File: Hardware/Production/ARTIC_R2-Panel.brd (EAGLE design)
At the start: 113 x 122.2 mm, 1045 parts, among them J1 U.FL, J10 U.FL, J11 THING_PLUS, J12 U.FL, J13 THING_PLUS, J14 U.FL, J15 THING_PLUS, J16 U.FL, J2 THING_PLUS, J3 THING_PLUS, J4 U.FL, J5 THING_PLUS, J6 U.FL, J7 THING_PLUS, J8 U.FL, J9 THING_PLUS, Q1 20V/4.2A/52mΩ/1.4W, Q2 20V/4.2A/52mΩ/1.4W, Q3 20V/4.2A/52mΩ/1.4W, Q4 20V/4.2A/52mΩ/1.4W, Q5 20V/4.2A/52mΩ/1.4W, Q6 20V/4.2A/52mΩ/1.4W, Q7 20V/4.2A/52mΩ/1.4W, Q8 20V/4.2A/52mΩ/1.4W, U1 32M SPI Flash, U10 1.8V/100mA, U11 32M SPI Flash, U12 DUAL-OPTOISOLATOR_SOIC8, U13 ARTIC_R2, U14 RFPA0133, U15 AS179-92LF, U16 1.8V/100mA, U17 32M SPI Flash, U18 DUAL-OPTOISOLATOR_SOIC8, U19 ARTIC_R2, U2 1.8V/100mA, U20 RFPA0133, U21 AS179-92LF, U22 1.8V/100mA, U23 32M SPI Flash, U24 DUAL-OPTOISOLATOR_SOIC8, U25 ARTIC_R2, U26 RFPA0133, U27 AS179-92LF, U28 1.8V/100mA, U29 32M SPI Flash, U3 ARTIC_R2, U30 DUAL-OPTOISOLATOR_SOIC8, U31 ARTIC_R2, U32 RFPA0133, U33 AS179-92LF, U34 1.8V/100mA, U35 32M SPI Flash, U36 DUAL-OPTOISOLATOR_SOIC8, U37 ARTIC_R2, U38 RFPA0133, U39 AS179-92LF, U4 RFPA0133, U40 1.8V/100mA, U41 32M SPI Flash, U42 DUAL-OPTOISOLATOR_SOIC8, U43 ARTIC_R2, U44 RFPA0133, U45 AS179-92LF, U46 1.8V/100mA, U47 32M SPI Flash, U48 DUAL-OPTOISOLATOR_SOIC8, U5 AS179-92LF, U6 DUAL-OPTOISOLATOR_SOIC8, U7 ARTIC_R2, U8 RFPA0133, U9 AS179-92LF, X1 CRYSTAL-TCXO-26MHZ, X2 CRYSTAL-TCXO-26MHZ, X3 CRYSTAL-TCXO-26MHZ, X4 CRYSTAL-TCXO-26MHZ, X5 CRYSTAL-TCXO-26MHZ, X6 CRYSTAL-TCXO-26MHZ, X7 CRYSTAL-TCXO-26MHZ, X8 CRYSTAL-TCXO-26MHZ

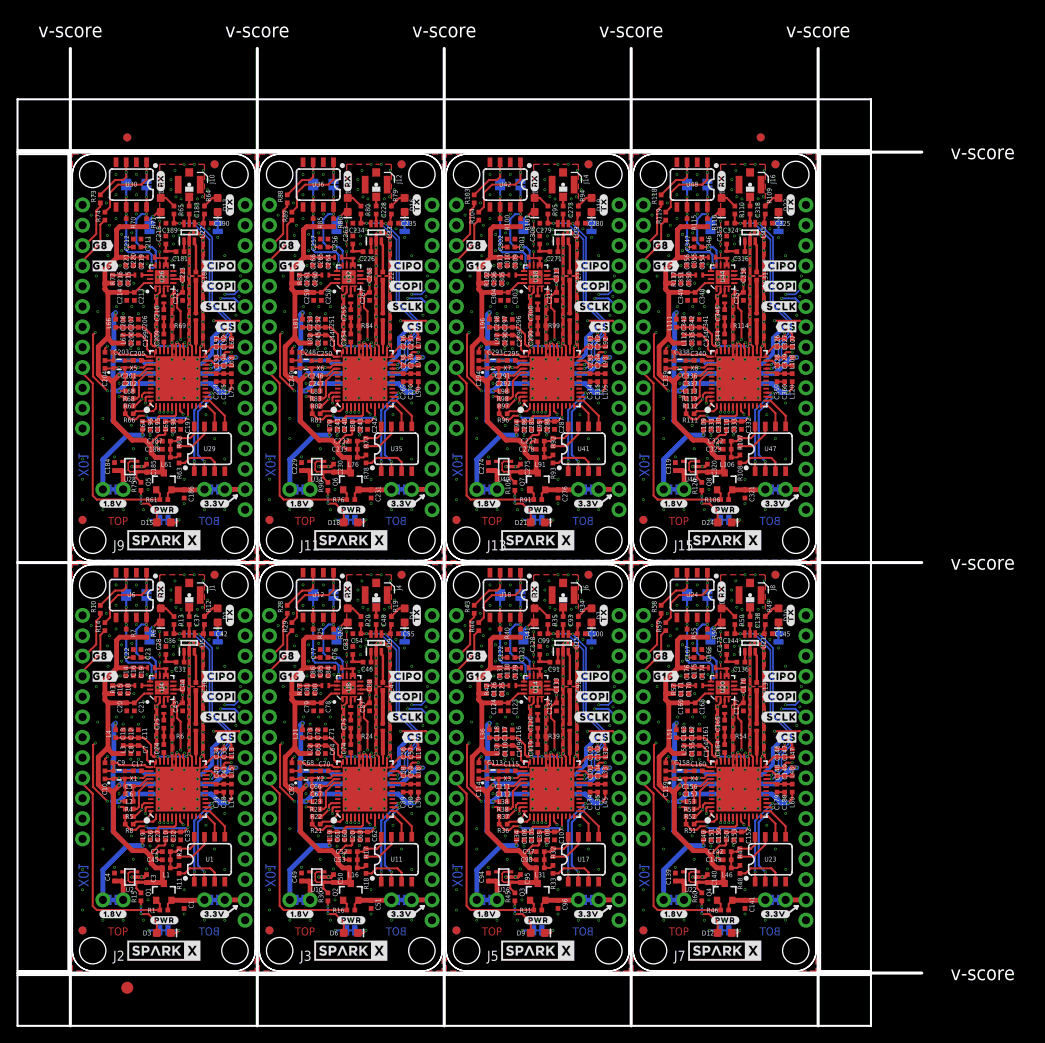
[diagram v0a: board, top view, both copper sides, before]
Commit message: Updates for X02
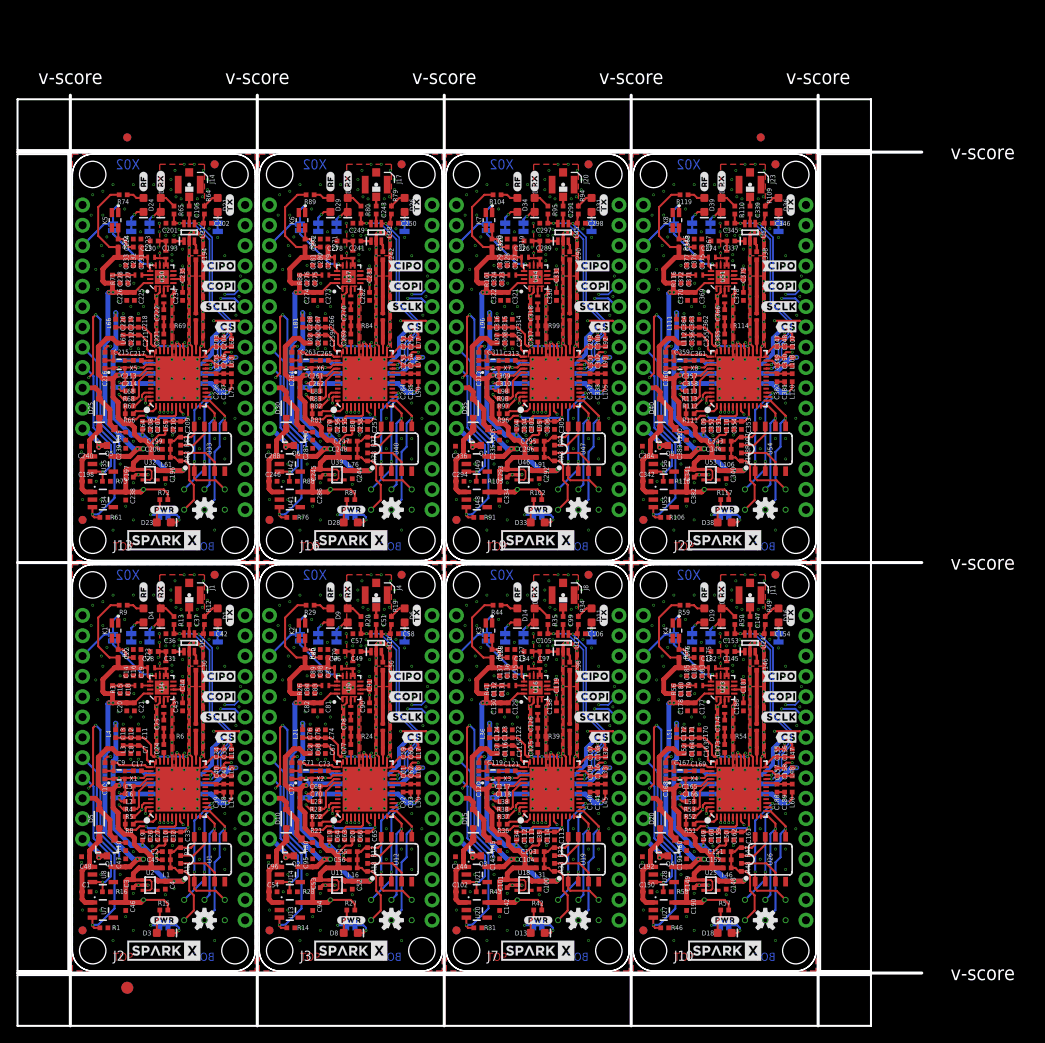
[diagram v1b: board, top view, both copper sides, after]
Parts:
- removed JP41, JP42, JP48, JP49, JP55, JP56: JUMPER-SMT_2_NO_SILK, SparkFun-Jumpers:SMT-JUMPER_2_NO_SILK
- removed JP43, JP44, JP50, JP51: JUMPER-COMBO_2_NC_TRACE, SparkFun-Jumpers:COMBO-JUMPER_2_NC_TRACE
- removed JP45, JP46, JP47, JP52, JP53, JP54: JUMPER-SMT_2_NC_TRACE_SILK, SparkFun-Jumpers:SMT-JUMPER_2_NC_TRACE_SILK
- removed U$225: (no value), output:#RESETB0
- removed U$226: (no value), output:#PWR_EN0
- removed U$227: (no value), output:GND#0
- removed U$228: (no value), output:#INT20
- removed U$229: (no value), output:#INT10
- removed U$230: (no value), output:#PWR_LED#0
- removed U$231: (no value), output:#PWR#0
- removed U$232: (no value), output:ARTIC_R2_BREAKOUT0
- added C361: 1.0nF, SparkFun-Capacitors:0402-TIGHT
- added C362, C365, C366, C367, C368, C369, C375, C378: 100pF, SparkFun-Capacitors:0402-TIGHT
- added C363: 1.0uF, SparkFun-Capacitors:0402-TIGHT
- added C364, C377: 10uF, SparkFun-Capacitors:0402-TIGHT
- added C370, C372, C376, C379, C382, C383: 2.2uF, SparkFun-Capacitors:0402-TIGHT
- added C371, C380: 22pF, SparkFun-Capacitors:0402-TIGHT
- added C373: 2.4 pF, SparkFun-Capacitors:0402_MURATA
- added C374: 9.1pF, New_Parts_Capacitors:0402-TIGHT
- added C381, C384: 0.1uF, SparkFun-Capacitors:0402-TIGHT
- added D25, D30, D35, D40: 1A/23V/620mV, SparkFun-DiscreteSemi:SOD-323
- added D26, D27, D31, D32, D36, D37: Yellow, SparkFun-LED:LED-0603
- added D28, D29, D33, D34, D38, D39: RED, SparkFun-LED:LED-0603
- added E$6: (no value), SparkFun-Retired:FIDUCIAL-1.5X3
- added J17, J20, J23: U.FL, SparkFun-Connectors:U.FL
- added J18, J21, J24: Flash Programming, SparkFun-Connectors:2X3_TEST_POINTS
- added J19, J22: THING_PLUS, New_Parts_Boards:THING_PLUS
- added K1, K2, K3, K4, K5, K6, K7, K8: TLP3475R, New_Parts_DiscreteSemi:TLP3475RTPF
- added LOGO1, LOGO10, LOGO11, LOGO12, LOGO13, LOGO14, LOGO15, LOGO16, LOGO2, LOGO3, LOGO4, LOGO5, LOGO6, LOGO7, LOGO8, LOGO9: OSHW-LOGOS, SparkFun-Aesthetics:OSHW-LOGO-S
- added TP1, TP10, TP11, TP12, TP13, TP14, TP15, TP16, TP17, TP18, TP19, TP2, TP20, TP21, TP22, TP23, TP24, TP3, TP4, TP5, TP6, TP7, TP8, TP9: TEST-POINTTP_15TH_THRU, SparkFun-Connectors:TP_15TH
- added U49, U55, U56: 3.3V, SparkFun-IC-Power:SOT23-5
- added U50: ARTIC_R2, New_Parts_IC-Comms:QFN-48
- added U51: RFPA0133, New_Parts_IC-Comms:QFN50P300X300X86-17N
- added U52: AS179-92LF, New_Parts_IC-Comms:SOT65P220X100-6N
- added U53: 1.8V/100mA, SparkFun-IC-Power:SC70
- added U54: 2Mbit SPI Flash, New_Parts_IC-Memory:SO08
- C1, C276: value 10uF -> 2.2uF
- C100, C119, C123, C167, C219, C267, C341, C71, C75: value 100pF -> 1.0uF
- C101, C148, C197, C215, C244, C359, C52: value 22pF -> 1.0uF
- C102, C143, C180, C198, C239, C286, C331, C335: value 0.1uF -> 2.2uF
- C105, C125, C146, C154, C170, C193, C195, C201, C224, C242, C269, C289, C291, C314, C330, C58, C80, C97: value 22pF -> 100pF
- C106, C135, C147, C153, C194, C202, C225, C241, C243, C270, C282, C290, C327, C337, C57, C90, C98: value 0.1uF -> 100pF
- C113, C117, C140, C203, C207, C275: value 1.0uF -> 22pF
- C114, C204: value 47nF -> 0.1uF
- C115, C205, C295: value 1.0nF -> 22pF
- C116, C144, C164, C166, C189, C206, C210, C212, C254, C256, C258, C296, C300, C302, C344, C348, C354, C48, C93: value 100pF -> 0.1uF
- C118, C141, C208, C356, C96: value 10uF -> 0.1uF
- C120, C168, C264, C312: value 100pF -> 47nF
- C121: value 100pF -> 1.0nF
- C124, C220, C268: value 2.2uF -> 10uF
- C126, C175, C223, C79, C81: value 2.2uF -> 100pF
- C127: value 2.4 pF -> 100pF; device SparkFun-Capacitors:0402_MURATA -> SparkFun-Capacitors:0402-TIGHT
- C128, C173, C218: value 9.1pF -> 100pF; device New_Parts_Capacitors:0402-TIGHT -> SparkFun-Capacitors:0402-TIGHT
- C131, C163, C253, C343: value 10uF -> 22pF
- C132, C136, C190, C226, C228, C235, C280, C324, C46, C47, C54, C84, C91: value 100pF -> 2.2uF
- C133, C85: value 2.2uF -> 2.4 pF; device SparkFun-Capacitors:0402-TIGHT -> SparkFun-Capacitors:0402_MURATA
- C134, C326: value 22pF -> 9.1pF; device SparkFun-Capacitors:0402-TIGHT -> New_Parts_Capacitors:0402-TIGHT
- C137, C316, C76: value 100pF -> 10uF
- C139, C184, C274, C342, C94, C95: value 1.0uF -> 2.2uF
- C142, C150, C187, C191, C232, C238, C246, C283, C287, C322, C328, C334: value 22pF -> 2.2uF
- C149, C196, C245, C292, C315, C53: value 0.1uF -> 1.0uF
- C151, C155, C157, C188, C247, C284, C323, C59, C61, C63, C65, C67: value 0.1uF -> 22pF
- C152, C156, C240, C260, C285, C336, C350, C56, C60, C62, C64, C66: value 22pF -> 0.1uF
- C158, C162, C248, C252, C68: value 1.0uF -> 0.1uF
- C159, C69: value 47nF -> 22pF
- C160, C70: value 1.0nF -> 0.1uF
- C161, C165, C209, C211, C213, C227, C251, C255, C257, C299, C301, C303, C309, C347, C357, C55, C92: value 100pF -> 22pF
- C169, C265, C313: value 2.2uF -> 1.0nF
- C171: value 2.2uF -> 1.0uF
- C172: value 2.4 pF -> 10uF; device SparkFun-Capacitors:0402_MURATA -> SparkFun-Capacitors:0402-TIGHT
- C176, C186, C221, C231, C266, C298, C321, C51: value 10uF -> 100pF
- C181, C325: value 100pF -> 2.4 pF; device SparkFun-Capacitors:0402-TIGHT -> SparkFun-Capacitors:0402_MURATA
- C182: value 100pF -> 9.1pF; device SparkFun-Capacitors:0402-TIGHT -> New_Parts_Capacitors:0402-TIGHT
- C185: value 1.0uF -> 10uF
- C214, C304, C306, C310, C358: value 2.2uF -> 0.1uF
- C216: value 2.2uF -> 47nF
- C217: value 2.4 pF -> 1.0nF; device SparkFun-Capacitors:0402_MURATA -> SparkFun-Capacitors:0402-TIGHT
- C229: value 1.0uF -> 2.4 pF; device SparkFun-Capacitors:0402-TIGHT -> SparkFun-Capacitors:0402_MURATA
- C230: value 1.0uF -> 9.1pF; device SparkFun-Capacitors:0402-TIGHT -> New_Parts_Capacitors:0402-TIGHT
- C233, C329: value 0.1uF -> 10uF
- C249, C339: value 47nF -> 100pF
- C250: value 1.0nF -> 100pF
- C259, C261, C349, C351, C355: value 2.2uF -> 22pF
- C262, C352: value 2.4 pF -> 0.1uF; device SparkFun-Capacitors:0402_MURATA -> SparkFun-Capacitors:0402-TIGHT
- C263: value 9.1pF -> 1.0uF; device New_Parts_Capacitors:0402-TIGHT -> SparkFun-Capacitors:0402-TIGHT
- C277: value 22pF -> 2.4 pF; device SparkFun-Capacitors:0402-TIGHT -> SparkFun-Capacitors:0402_MURATA
- C278: value 0.1uF -> 9.1pF; device SparkFun-Capacitors:0402-TIGHT -> New_Parts_Capacitors:0402-TIGHT
- C281, C89: value 22pF -> 10uF
- C294: value 47nF -> 2.2uF
- C297, C319, C320, C338, C49, C50: value 1.0uF -> 100pF
- C307: value 2.4 pF -> 22pF; device SparkFun-Capacitors:0402_MURATA -> SparkFun-Capacitors:0402-TIGHT
- C308: value 9.1pF -> 0.1uF; device New_Parts_Capacitors:0402-TIGHT -> SparkFun-Capacitors:0402-TIGHT
- C311: value 10uF -> 1.0uF
- C340: value 1.0nF -> 1.0uF
- C353, C83: value 9.1pF -> 22pF; device New_Parts_Capacitors:0402-TIGHT -> SparkFun-Capacitors:0402-TIGHT
- C360: value 0.1uF -> 47nF
- C72: value 1.0uF -> 47nF
- C73: value 10uF -> 1.0nF
- C82: value 2.4 pF -> 2.2uF; device SparkFun-Capacitors:0402_MURATA -> SparkFun-Capacitors:0402-TIGHT
- C86: value 10uF -> 9.1pF; device SparkFun-Capacitors:0402-TIGHT -> New_Parts_Capacitors:0402-TIGHT
- D10, D20, D5: value Yellow -> 1A/23V/620mV; device SparkFun-LED:LED-0603 -> SparkFun-DiscreteSemi:SOD-323
- D12, D21, D6: value RED -> Yellow
- D13, D14, D19, D23, D4, D8: value Yellow -> RED
- D15: value RED -> 1A/23V/620mV; device SparkFun-LED:LED-0603 -> SparkFun-DiscreteSemi:SOD-323
- J10, J16: value U.FL -> THING_PLUS; device SparkFun-Connectors:U.FL -> New_Parts_Boards:THING_PLUS
- J11: value THING_PLUS -> U.FL; device New_Parts_Boards:THING_PLUS -> SparkFun-Connectors:U.FL
- J12, J6: value U.FL -> Flash Programming; device SparkFun-Connectors:U.FL -> SparkFun-Connectors:2X3_TEST_POINTS
- J15, J5, J9: value THING_PLUS -> Flash Programming; device New_Parts_Boards:THING_PLUS -> SparkFun-Connectors:2X3_TEST_POINTS
- JP1, JP15, JP16, JP2, JP22, JP23, JP30, JP36, JP37, JP8: value JUMPER-COMBO_2_NC_TRACE -> JUMPER-SMT_2_NC_TRACE_SILK; device SparkFun-Jumpers:COMBO-JUMPER_2_NC_TRACE -> SparkFun-Jumpers:SMT-JUMPER_2_NC_TRACE_SILK
- JP13, JP20, JP21, JP27, JP28, JP35, JP6: value JUMPER-SMT_2_NO_SILK -> JUMPER-SMT_2_NC_TRACE_SILK; device SparkFun-Jumpers:SMT-JUMPER_2_NO_SILK -> SparkFun-Jumpers:SMT-JUMPER_2_NC_TRACE_SILK
- JP19, JP24, JP39: value JUMPER-SMT_2_NC_TRACE_SILK -> JUMPER-SMT_2_NO_SILK; device SparkFun-Jumpers:SMT-JUMPER_2_NC_TRACE_SILK -> SparkFun-Jumpers:SMT-JUMPER_2_NO_SILK
- JP29, JP9: value JUMPER-COMBO_2_NC_TRACE -> JUMPER-SMT_2_NO_SILK; device SparkFun-Jumpers:COMBO-JUMPER_2_NC_TRACE -> SparkFun-Jumpers:SMT-JUMPER_2_NO_SILK
- Q1, Q2, Q3, Q4, Q5, Q6, Q7, Q8: value 20V/4.2A/52mΩ/1.4W -> 3.1A/30V/105mΩ
- R10, R103, R105, R118, R120, R14, R28, R30, R43, R45, R58, R60, R73, R75, R88, R90: value 1k -> 100k
- R100, R115, R25, R40, R55, R7, R70, R85: value 100k -> 10k
- R101, R116, R26, R41, R56, R71, R86: value 100k -> 3.9OHM; device SparkFun-Resistors:0402-TIGHT -> New_Parts_Resistors:0402-TIGHT
- R102, R117, R27, R42, R57, R72, R87: value 3.9OHM -> 1k; device New_Parts_Resistors:0402-TIGHT -> SparkFun-Resistors:0402-TIGHT
- R9: value 100k -> 1k
- U$100: device output:#SCLK0 -> output:GND#0
- U$101: device output:SCLK#0 -> output:#INT20
- U$102: device output:#CS0 -> output:#INT10
- U$103: device output:CS#0 -> output:#PWR_LED#0
- U$104: device output:G8#0 -> output:#PWR#0
- U$105: device output:#G80 -> output:ARTIC_R2_BREAKOUT0
- U$106: device output:G16#0 -> output:#RF_LED#0
- U$107: device output:#G160 -> output:#GAIN8#0
- U$108: device output:#BOOT0 -> output:#RF#0
- U$109: device output:#RESETB0 -> output:#RF_EN#0
- U$110: device output:#PWR_EN0 -> output:#VBATT#0
- U$111: device output:GND#0 -> output:##8DB#0
- U$112: device output:#INT20 -> output:#VUSB#0
- U$113: device output:#INT10 -> output:#RX_LED#0
- U$114: device output:#PWR_LED#0 -> output:#TX_LED#0
- U$115: device output:#PWR#0 -> output:#TX#0
- U$116: device output:ARTIC_R2_BREAKOUT0 -> output:#RX#0
- U$117: device output:#RX_LED#0 -> output:CIPO#0
- U$118: device output:#TX_LED#0 -> output:#CIPO0
- U$119, U$91: device output:#3#3V#0 -> output:#COPI0
- U$120, U$148: device output:#3#3V#0 -> output:COPI#0
- U$121, U$93: device output:#1#8V#0 -> output:#SCLK0
- U$122, U$150: device output:#1#8V#0 -> output:SCLK#0
- U$123: device output:#TX#0 -> output:#CS0
- U$124: device output:#RX#0 -> output:CS#0
- U$125: device output:CIPO#0 -> output:#BOOT0
- U$126: device output:#CIPO0 -> output:#RESETB0
- U$127: device output:#COPI0 -> output:#PWR_EN0
- U$128: device output:COPI#0 -> output:GND#0
- U$129: device output:#SCLK0 -> output:#INT20
- U$130: device output:SCLK#0 -> output:#INT10
- U$131: device output:#CS0 -> output:#PWR_LED#0
- U$132: device output:CS#0 -> output:#PWR#0
- U$133: device output:G8#0 -> output:ARTIC_R2_BREAKOUT0
- U$134: device output:#G80 -> output:#RF_LED#0
- U$135: device output:G16#0 -> output:#GAIN8#0
- U$136: device output:#G160 -> output:#RF#0
- U$137: device output:#BOOT0 -> output:#RF_EN#0
- U$138: device output:#RESETB0 -> output:#VBATT#0
- U$139: device output:#PWR_EN0 -> output:##8DB#0
- U$140: device output:GND#0 -> output:#VUSB#0
- U$141: device output:#INT20 -> output:#RX_LED#0
- U$142: device output:#INT10 -> output:#TX_LED#0
- U$143: device output:#PWR_LED#0 -> output:#TX#0
- U$144: device output:#PWR#0 -> output:#RX#0
- U$145: device output:ARTIC_R2_BREAKOUT0 -> output:CIPO#0
- U$146: device output:#RX_LED#0 -> output:#CIPO0
- U$147: device output:#TX_LED#0 -> output:#COPI0
- U$149, U$177: device output:#3#3V#0 -> output:#SCLK0
- U$151, U$179: device output:#1#8V#0 -> output:#CS0
- U$152: device output:#TX#0 -> output:CS#0
- U$153: device output:#RX#0 -> output:#BOOT0
- U$154: device output:CIPO#0 -> output:#RESETB0
- U$155: device output:#CIPO0 -> output:#PWR_EN0
- U$156: device output:#COPI0 -> output:GND#0
- U$157: device output:COPI#0 -> output:#INT20
- U$158: device output:#SCLK0 -> output:#INT10
- U$159: device output:SCLK#0 -> output:#PWR_LED#0
- U$160: device output:#CS0 -> output:#PWR#0
- U$161: device output:CS#0 -> output:ARTIC_R2_BREAKOUT0
- U$162: device output:G8#0 -> output:#RF_LED#0
- U$163: device output:#G80 -> output:#GAIN8#0
- U$164: device output:G16#0 -> output:#RF#0
- U$165: device output:#G160 -> output:#RF_EN#0
- U$166: device output:#BOOT0 -> output:#VBATT#0
- U$167: device output:#RESETB0 -> output:##8DB#0
- U$168: device output:#PWR_EN0 -> output:#VUSB#0
- U$169: device output:GND#0 -> output:#RX_LED#0
- U$170: device output:#INT20 -> output:#TX_LED#0
- U$171: device output:#INT10 -> output:#TX#0
- U$172: device output:#PWR_LED#0 -> output:#RX#0
- U$173: device output:#PWR#0 -> output:CIPO#0
- U$174: device output:ARTIC_R2_BREAKOUT0 -> output:#CIPO0
- U$175: device output:#RX_LED#0 -> output:#COPI0
- U$176: device output:#TX_LED#0 -> output:COPI#0
- U$178, U$206: device output:#3#3V#0 -> output:SCLK#0
- U$180, U$208: device output:#1#8V#0 -> output:CS#0
- U$181: device output:#TX#0 -> output:#BOOT0
- U$182: device output:#RX#0 -> output:#RESETB0
- U$183: device output:CIPO#0 -> output:#PWR_EN0
- U$184: device output:#CIPO0 -> output:GND#0
- U$185: device output:#COPI0 -> output:#INT20
- U$186: device output:COPI#0 -> output:#INT10
- U$187: device output:#SCLK0 -> output:#PWR_LED#0
- U$188: device output:SCLK#0 -> output:#PWR#0
- U$189: device output:#CS0 -> output:ARTIC_R2_BREAKOUT0
- U$190: device output:CS#0 -> output:#RF_LED#0
- U$191: device output:G8#0 -> output:#GAIN8#0
- U$192: device output:#G80 -> output:#RF#0
- U$193: device output:G16#0 -> output:#RF_EN#0
- U$194: device output:#G160 -> output:#VBATT#0
- U$195: device output:#BOOT0 -> output:##8DB#0
- U$196: device output:#RESETB0 -> output:#VUSB#0
- U$197: device output:#PWR_EN0 -> output:#RX_LED#0
- U$198: device output:GND#0 -> output:#TX_LED#0
- U$199: device output:#INT20 -> output:#TX#0
- U$20: device output:G8#0 -> output:#VBATT#0
- U$200: device output:#INT10 -> output:#RX#0
- U$201: device output:#PWR_LED#0 -> output:CIPO#0
- U$202: device output:#PWR#0 -> output:#CIPO0
- U$203: device output:ARTIC_R2_BREAKOUT0 -> output:#COPI0
- U$204: device output:#RX_LED#0 -> output:COPI#0
- U$205: device output:#TX_LED#0 -> output:#SCLK0
- U$207: device output:#3#3V#0 -> output:#CS0
- U$209: device output:#1#8V#0 -> output:#BOOT0
- U$21: device output:#G80 -> output:#VUSB#0
- U$210: device output:#TX#0 -> output:#RESETB0
- U$211: device output:#RX#0 -> output:#PWR_EN0
- U$212: device output:CIPO#0 -> output:GND#0
- U$213: device output:#CIPO0 -> output:#INT20
- U$214: device output:#COPI0 -> output:#INT10
- U$215: device output:COPI#0 -> output:#PWR_LED#0
- U$216: device output:#SCLK0 -> output:#PWR#0
- U$217: device output:SCLK#0 -> output:ARTIC_R2_BREAKOUT0
- U$218: device output:#CS0 -> output:#RF_LED#0
- U$219: device output:CS#0 -> output:#GAIN8#0
- U$22: device output:G16#0 -> output:##8DB#0
- U$220: device output:G8#0 -> output:#RF#0
- U$221: device output:#G80 -> output:#RF_EN#0
- U$222: device output:G16#0 -> output:#VBATT#0
- U$223: device output:#G160 -> output:##8DB#0
- U$224: device output:#BOOT0 -> output:#VUSB#0
- U$23: device output:#G160 -> output:#RX_LED#0
- U$30: device output:#RX_LED#0 -> output:#TX_LED#0
- U$31: device output:#TX_LED#0 -> output:#TX#0
- U$32: device output:#3#3V#0 -> output:#RX#0
- U$33, U$61: device output:#3#3V#0 -> output:CIPO#0
- U$34: device output:#1#8V#0 -> output:#CIPO0
- U$35, U$63: device output:#1#8V#0 -> output:#COPI0
- U$36: device output:#TX#0 -> output:COPI#0
- U$37: device output:#RX#0 -> output:#SCLK0
- U$38: device output:CIPO#0 -> output:SCLK#0
- U$39: device output:#CIPO0 -> output:#CS0
- U$40: device output:#COPI0 -> output:CS#0
- U$41: device output:COPI#0 -> output:#BOOT0
- U$42: device output:#SCLK0 -> output:#RESETB0
- U$43: device output:SCLK#0 -> output:#PWR_EN0
- U$44: device output:#CS0 -> output:GND#0
- U$45: device output:CS#0 -> output:#INT20
- U$46: device output:G8#0 -> output:#INT10
- U$47: device output:#G80 -> output:#PWR_LED#0
- U$48: device output:G16#0 -> output:#PWR#0
- U$49: device output:#G160 -> output:ARTIC_R2_BREAKOUT0
- U$5: device output:#3#3V#0 -> output:#RF_LED#0
- U$50: device output:#BOOT0 -> output:#RF_LED#0
- U$51: device output:#RESETB0 -> output:#GAIN8#0
- U$52: device output:#PWR_EN0 -> output:#RF#0
- U$53: device output:GND#0 -> output:#RF_EN#0
- U$54: device output:#INT20 -> output:#VBATT#0
- U$55: device output:#INT10 -> output:##8DB#0
- U$56: device output:#PWR_LED#0 -> output:#VUSB#0
- U$57: device output:#PWR#0 -> output:#RX_LED#0
- U$58: device output:ARTIC_R2_BREAKOUT0 -> output:#TX_LED#0
- U$59: device output:#RX_LED#0 -> output:#TX#0
- U$6: device output:#3#3V#0 -> output:#GAIN8#0
- U$60: device output:#TX_LED#0 -> output:#RX#0
- U$62, U$90: device output:#3#3V#0 -> output:#CIPO0
- U$64, U$92: device output:#1#8V#0 -> output:COPI#0
- U$65: device output:#TX#0 -> output:#SCLK0
- U$66: device output:#RX#0 -> output:SCLK#0
- U$67: device output:CIPO#0 -> output:#CS0
- U$68: device output:#CIPO0 -> output:CS#0
- U$69: device output:#COPI0 -> output:#BOOT0
- U$7: device output:#1#8V#0 -> output:#RF#0
- U$70: device output:COPI#0 -> output:#RESETB0
- U$71: device output:#SCLK0 -> output:#PWR_EN0
- U$72: device output:SCLK#0 -> output:GND#0
- U$73: device output:#CS0 -> output:#INT20
- U$74: device output:CS#0 -> output:#INT10
- U$75: device output:G8#0 -> output:#PWR_LED#0
- U$76: device output:#G80 -> output:#PWR#0
- U$77: device output:G16#0 -> output:ARTIC_R2_BREAKOUT0
- U$78: device output:#G160 -> output:#RF_LED#0
- U$79: device output:#BOOT0 -> output:#GAIN8#0
- U$8: device output:#1#8V#0 -> output:#RF_EN#0
- U$80: device output:#RESETB0 -> output:#RF#0
- U$81: device output:#PWR_EN0 -> output:#RF_EN#0
- U$82: device output:GND#0 -> output:#VBATT#0
- U$83: device output:#INT20 -> output:##8DB#0
- U$84: device output:#INT10 -> output:#VUSB#0
- U$85: device output:#PWR_LED#0 -> output:#RX_LED#0
- U$86: device output:#PWR#0 -> output:#TX_LED#0
- U$87: device output:ARTIC_R2_BREAKOUT0 -> output:#TX#0
- U$88: device output:#RX_LED#0 -> output:#RX#0
- U$89: device output:#TX_LED#0 -> output:CIPO#0
- U$94: device output:#TX#0 -> output:SCLK#0
- U$95: device output:#RX#0 -> output:#CS0
- U$96: device output:CIPO#0 -> output:CS#0
- U$97: device output:#CIPO0 -> output:#BOOT0
- U$98: device output:#COPI0 -> output:#RESETB0
- U$99: device output:COPI#0 -> output:#PWR_EN0
- U1, U47: value 32M SPI Flash -> 2Mbit SPI Flash; device SparkFun-IC-Memory:SO08 -> New_Parts_IC-Memory:SO08
- U10: value 1.8V/100mA -> AS179-92LF; device SparkFun-IC-Power:SC70 -> New_Parts_IC-Comms:SOT65P220X100-6N
- U11: value 32M SPI Flash -> 1.8V/100mA; device SparkFun-IC-Memory:SO08 -> SparkFun-IC-Power:SC70
- U12: value DUAL-OPTOISOLATOR_SOIC8 -> 2Mbit SPI Flash; device SparkFun-DiscreteSemi:SO08 -> New_Parts_IC-Memory:SO08
- U13, U7: value ARTIC_R2 -> 3.3V; device New_Parts_IC-Comms:QFN-48 -> SparkFun-IC-Power:SOT23-5
- U14, U20, U8: value RFPA0133 -> 3.3V; device New_Parts_IC-Comms:QFN50P300X300X86-17N -> SparkFun-IC-Power:SOT23-5
- U15: value AS179-92LF -> ARTIC_R2; device New_Parts_IC-Comms:SOT65P220X100-6N -> New_Parts_IC-Comms:QFN-48
- U16: value 1.8V/100mA -> RFPA0133; device SparkFun-IC-Power:SC70 -> New_Parts_IC-Comms:QFN50P300X300X86-17N
- U17: value 32M SPI Flash -> AS179-92LF; device SparkFun-IC-Memory:SO08 -> New_Parts_IC-Comms:SOT65P220X100-6N
- U18: value DUAL-OPTOISOLATOR_SOIC8 -> 1.8V/100mA; device SparkFun-DiscreteSemi:SO08 -> SparkFun-IC-Power:SC70
- U19: value ARTIC_R2 -> 2Mbit SPI Flash; device New_Parts_IC-Comms:QFN-48 -> New_Parts_IC-Memory:SO08
- U21, U27: value AS179-92LF -> 3.3V; device New_Parts_IC-Comms:SOT65P220X100-6N -> SparkFun-IC-Power:SOT23-5
- U22: value 1.8V/100mA -> ARTIC_R2; device SparkFun-IC-Power:SC70 -> New_Parts_IC-Comms:QFN-48
- U23: value 32M SPI Flash -> RFPA0133; device SparkFun-IC-Memory:SO08 -> New_Parts_IC-Comms:QFN50P300X300X86-17N
- U24: value DUAL-OPTOISOLATOR_SOIC8 -> AS179-92LF; device SparkFun-DiscreteSemi:SO08 -> New_Parts_IC-Comms:SOT65P220X100-6N
- U25: value ARTIC_R2 -> 1.8V/100mA; device New_Parts_IC-Comms:QFN-48 -> SparkFun-IC-Power:SC70
- U26: value RFPA0133 -> 2Mbit SPI Flash; device New_Parts_IC-Comms:QFN50P300X300X86-17N -> New_Parts_IC-Memory:SO08
- U28, U34: value 1.8V/100mA -> 3.3V; device SparkFun-IC-Power:SC70 -> SparkFun-IC-Power:SOT23-5
- U29: value 32M SPI Flash -> ARTIC_R2; device SparkFun-IC-Memory:SO08 -> New_Parts_IC-Comms:QFN-48
- U30: value DUAL-OPTOISOLATOR_SOIC8 -> RFPA0133; device SparkFun-DiscreteSemi:SO08 -> New_Parts_IC-Comms:QFN50P300X300X86-17N
- U31: value ARTIC_R2 -> AS179-92LF; device New_Parts_IC-Comms:QFN-48 -> New_Parts_IC-Comms:SOT65P220X100-6N
- U32: value RFPA0133 -> 1.8V/100mA; device New_Parts_IC-Comms:QFN50P300X300X86-17N -> SparkFun-IC-Power:SC70
- U33: value AS179-92LF -> 2Mbit SPI Flash; device New_Parts_IC-Comms:SOT65P220X100-6N -> New_Parts_IC-Memory:SO08
- U35, U41: value 32M SPI Flash -> 3.3V; device SparkFun-IC-Memory:SO08 -> SparkFun-IC-Power:SOT23-5
- U36, U6: value DUAL-OPTOISOLATOR_SOIC8 -> ARTIC_R2; device SparkFun-DiscreteSemi:SO08 -> New_Parts_IC-Comms:QFN-48
- U37: value ARTIC_R2 -> RFPA0133; device New_Parts_IC-Comms:QFN-48 -> New_Parts_IC-Comms:QFN50P300X300X86-17N
- U38: value RFPA0133 -> AS179-92LF; device New_Parts_IC-Comms:QFN50P300X300X86-17N -> New_Parts_IC-Comms:SOT65P220X100-6N
- U39: value AS179-92LF -> 1.8V/100mA; device New_Parts_IC-Comms:SOT65P220X100-6N -> SparkFun-IC-Power:SC70
- U40: value 1.8V/100mA -> 2Mbit SPI Flash; device SparkFun-IC-Power:SC70 -> New_Parts_IC-Memory:SO08
- U42, U48: value DUAL-OPTOISOLATOR_SOIC8 -> 3.3V; device SparkFun-DiscreteSemi:SO08 -> SparkFun-IC-Power:SOT23-5
- U9: value AS179-92LF -> RFPA0133; device New_Parts_IC-Comms:SOT65P220X100-6N -> New_Parts_IC-Comms:QFN50P300X300X86-17N
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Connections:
- removed net 3.3V: C1.1, JP1.2, JP1.4, Q1.2, R1.2
- removed net 3.3V1: C51.1, JP8.2, JP8.4, Q2.2, R16.2
- removed net 3.3V2: C96.1, JP15.2, JP15.4, Q3.2, R31.2
- removed net 3.3V3: C141.1, JP22.2, JP22.4, Q4.2, R46.2
- removed net 3.3V4: C186.1, JP29.2, JP29.4, Q5.2, R61.2
- removed net 3.3V5: C231.1, JP36.2, JP36.4, Q6.2, R76.2
- removed net 3.3V6: C276.1, JP43.2, JP43.4, Q7.2, R91.2
- removed net 3.3V7: C321.1, JP50.2, JP50.4, Q8.2, R106.2
- removed net G10: J11.4, R89.2
- removed net G11: J11.3, R88.1
- removed net G12: J13.4, R104.2
- removed net G13: J13.3, R103.1
- removed net G14: J15.4, R119.2
- removed net G15: J15.3, R118.1
- removed net G16: J2.4, R14.2
- removed net G9: J9.3, R73.1
- removed net N$265: C341.1, C342.1, C343.1, L111.1, U43.28, U43.33, U43.35
- removed net N$266: C334.1, C335.1, L112.1, U43.36
- removed net N$267: R113.1, U43.41
- removed net N$268: C336.1, C337.1, L113.1, U43.40
- removed net N$269: C338.1, C339.1, U43.37, X8.4
- removed net N$270: C340.1, X8.3
- removed net N$271: C340.2, U43.38
- removed net N$272: C344.1, U43.34
- removed net N$273: C344.2, C345.1, R114.2
- removed net N$274: L115.P$2, U44.14
- removed net N$275: C350.1, C351.1, L115.P$1, R117.1
- removed net N$276: C345.2, L114.P$1
- removed net N$277: L114.P$2, U44.3
- removed net N$278: L116.P$2, L117.P$1, U44.10, U44.9
- removed net N$279: C352.P$1, L118.P$2, U43.26
- removed net N$280: J15.27, JP50.1, JP50.3
- removed net N$281: JP56.1, R118.2, U48.3
- removed net N$282: JP55.1, R119.1, U48.1
- removed net N$283: C359.1, C360.1, L120.1, U43.20
- removed net N$284: C319.1, JP51.1, JP51.3, U46.5
- removed net N$285: D22.C, JP52.2
- removed net N$286: D23.C, JP53.2
- removed net N$287: D24.A, R120.1
- removed net N$288: D24.C, JP54.2
- removed net PWR_EN: J2.9, Q1.1, R1.1
- removed net PWR_EN1: J3.9, Q2.1, R16.1
- removed net PWR_EN2: J5.9, Q3.1, R31.1
- removed net PWR_EN3: J7.9, Q4.1, R46.1
- removed net PWR_EN4: J9.9, Q5.1, R61.1
- removed net PWR_EN5: J11.9, Q6.1, R76.1
- removed net PWR_EN6: J13.9, Q7.1, R91.1
- removed net PWR_EN7: J15.9, Q8.1, R106.1
- removed net RFG10: C256.2, JP41.2, R86.1, U32.13, U36.8
- removed net RFG11: C257.2, JP42.2, R85.1, U32.12, U36.6
- removed net RFG12: C301.2, JP48.2, R101.1, U38.13, U42.8
- removed net RFG13: C302.2, JP49.2, R100.1, U38.12, U42.6
- removed net RFG14: C346.2, JP55.2, R116.1, U44.13, U48.8
- removed net RFG15: C347.2, JP56.2, R115.1, U44.12, U48.6
- removed net RFG16: C23.2, JP6.2, R9.1, U4.13, U6.8
- removed net RFG9: C212.2, JP35.2, R70.1, U26.12, U30.6
- new net ARTIC_PWR_EN: J2.8, R1.2, U7.3
- new net ARTIC_PWR_EN1: J3.8, R14.2, U13.3
- new net ARTIC_PWR_EN2: J7.8, R31.2, U20.3
- new net ARTIC_PWR_EN3: J10.8, R46.2, U27.3
- new net ARTIC_PWR_EN4: J13.8, R61.2, U34.3
- new net ARTIC_PWR_EN5: J16.8, R76.2, U41.3
- new net ARTIC_PWR_EN6: J19.8, R91.2, U48.3
- new net ARTIC_PWR_EN7: J22.8, R106.2, U55.3
- new net FLSH_VCC: C2.1, C45.1, J5.2, L1.1, R11.2, R2.2, U1.8
- new net FLSH_VCC1: C55.1, C56.1, J6.2, L16.1, R17.2, R18.2, U12.8
- new net FLSH_VCC2: C103.1, C104.1, J9.2, L31.1, R32.2, R33.2, U19.8
- new net FLSH_VCC3: C151.1, C152.1, J12.2, L46.1, R47.2, R48.2, U26.8
- new net FLSH_VCC4: C199.1, C200.1, J15.2, L61.1, R62.2, R63.2, U33.8
- new net FLSH_VCC5: C247.1, C248.1, J18.2, L76.1, R77.2, R78.2, U40.8
- new net FLSH_VCC6: C295.1, C296.1, J21.2, L91.1, R92.2, R93.2, U47.8
- new net FLSH_VCC7: C343.1, C344.1, J24.2, L106.1, R107.2, R108.2, U54.8
- new net RF_PWR_EN: J2.9, R16.2, U8.3
- new net RF_PWR_EN1: J3.9, R28.2, U14.3
- new net RF_PWR_EN2: J7.9, R43.2, U21.3
- new net RF_PWR_EN3: J10.9, R58.2, U28.3
- new net RF_PWR_EN4: J13.9, R73.2, U35.3
- new net RF_PWR_EN5: J16.9, R88.2, U42.3
- new net RF_PWR_EN6: J19.9, R103.2, U49.3
- new net RF_PWR_EN7: J22.9, R118.2, U56.3
- new net VDDA: C14.1, C16.1, C19.1, C20.2, C21.2, C23.2, C47.1, L6.P$1, R3.2, R7.2, R9.2, TP2.P$1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
- new net VDDA1: C79.2, C81.2, C82.2, C87.1, C88.1, C89.1, C95.1, L26.P$1, R25.2, R26.2, R29.2, TP5.P$1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
- new net VDDA2: C127.2, C129.2, C130.2, C135.1, C136.1, C137.1, C143.1, L41.P$1, R40.2, R41.2, R44.2, TP8.P$1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
- new net VDDA3: C175.2, C177.2, C178.2, C183.1, C184.1, C185.1, C191.1, L56.P$1, R55.2, R56.2, R59.2, TP11.P$1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
- new net VDDA4: C223.2, C225.2, C226.2, C231.1, C232.1, C233.1, C239.1, L71.P$1, R70.2, R71.2, R74.2, TP14.P$1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
- new net VDDA5: C271.2, C273.2, C274.2, C279.1, C280.1, C281.1, C287.1, L86.P$1, R85.2, R86.2, R89.2, TP17.P$1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
- new net VDDA6: C319.2, C321.2, C322.2, C327.1, C328.1, C329.1, C335.1, L101.P$1, R100.2, R101.2, R104.2, TP20.P$1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
- new net VDDA7: C367.2, C369.2, C370.2, C375.1, C376.1, C377.1, C383.1, L116.P$1, R115.2, R116.2, R119.2, TP23.P$1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
- new net VIN: C1.1, C48.1, D5.C, Q1.2, U7.1, U8.1
- new net VIN1: C54.1, C96.1, D10.C, Q2.2, U13.1, U14.1
- new net VIN2: C102.1, C144.1, D15.C, Q3.2, U20.1, U21.1
- new net VIN3: C150.1, C192.1, D20.C, Q4.2, U27.1, U28.1
- new net VIN4: C198.1, C240.1, D25.C, Q5.2, U34.1, U35.1
- new net VIN5: C246.1, C288.1, D30.C, Q6.2, U41.1, U42.1
- new net VIN6: C294.1, C336.1, D35.C, Q7.2, U48.1, U49.1
- new net VIN7: C342.1, C384.1, D40.C, Q8.2, U55.1, U56.1
- new net V_BATT: J2.12, Q1.3
- new net V_BATT1: J3.12, Q2.3
- new net V_BATT2: J7.12, Q3.3
- new net V_BATT3: J10.12, Q4.3
- new net V_BATT4: J13.12, Q5.3
- new net V_BATT5: J16.12, Q6.3
- new net V_BATT6: J19.12, Q7.3
- new net V_BATT7: J22.12, Q8.3
- new net V_USB: D5.A, J2.10, Q1.1, R10.2
- new net V_USB1: D10.A, J3.10, Q2.1, R30.2
- new net V_USB2: D15.A, J7.10, Q3.1, R45.2
- new net V_USB3: D20.A, J10.10, Q4.1, R60.2
- new net V_USB4: D25.A, J13.10, Q5.1, R75.2
- new net V_USB5: D30.A, J16.10, Q6.1, R90.2
- new net V_USB6: D35.A, J19.10, Q7.1, R105.2
- new net V_USB7: D40.A, J22.10, Q8.1, R120.2
- net 1.8V: now also C4.1, TP3.P$1, U2.5; no longer JP2.2, JP2.4
- net 1.8V1: now also C52.1, TP6.P$1, U11.5; no longer JP9.2, JP9.4
- net 1.8V2: now also C100.1, TP9.P$1, U18.5; no longer JP16.2, JP16.4
- net 1.8V3: now also C148.1, TP12.P$1, U25.5; no longer JP23.2, JP23.4
- net 1.8V4: now also C196.1, TP15.P$1, U32.5; no longer JP30.2, JP30.4
- net 1.8V5: now also C244.1, TP18.P$1, U39.5; no longer JP37.2, JP37.4
- net 1.8V6: now also C292.1, TP21.P$1, U46.5; no longer JP44.2, JP44.4
- net 1.8V7: now also C340.1, TP24.P$1, U53.5; no longer JP51.2, JP51.4
- net ANTENNA1: now also C51.1; no longer C48.1
- net ANTENNA2: now also C99.1, J8.FEED; no longer C93.1, J6.FEED
- net ANTENNA3: now also C147.1, J11.FEED; no longer C138.1, J8.FEED
- net ANTENNA4: now also C195.1, J14.FEED; no longer C183.1, J10.FEED
- net ANTENNA5: now also C243.1, J17.FEED; no longer C228.1, J12.FEED
- net ANTENNA6: now also C291.1, J20.FEED; no longer C273.1, J14.FEED
- net ANTENNA7: now also C339.1, J23.FEED; no longer C318.1, J16.FEED
- net BOOT: now also J2.4; no longer J2.5
- net BOOT1: now also J3.4, U6.46; no longer J3.5, U7.46
- net BOOT2: now also J7.4, U15.46; no longer J5.5, U13.46
- net BOOT3: now also J10.4, U22.46; no longer J7.5, U19.46
- net BOOT4: now also J13.4, U29.46; no longer J9.5, U25.46
- net BOOT5: now also J16.4, U36.46; no longer J11.5, U31.46
- net BOOT6: now also J19.4, U43.46; no longer J13.5, U37.46
- net BOOT7: now also J22.4, U50.46; no longer J15.5, U43.46
- net CIPO1: now also U6.5; no longer U7.5
- net CIPO2: now also J7.16, U15.5; no longer J5.16, U13.5
- net CIPO3: now also J10.16, U22.5; no longer J7.16, U19.5
- net CIPO4: now also J13.16, U29.5; no longer J9.16, U25.5
- net CIPO5: now also J16.16, U36.5; no longer J11.16, U31.5
- net CIPO6: now also J19.16, U43.5; no longer J13.16, U37.5
- net CIPO7: now also J22.16, U50.5; no longer J15.16, U43.5
- net COPI1: now also U6.4; no longer U7.4
- net COPI2: now also J7.17, U15.4; no longer J5.17, U13.4
- net COPI3: now also J10.17, U22.4; no longer J7.17, U19.4
- net COPI4: now also J13.17, U29.4; no longer J9.17, U25.4
- net COPI5: now also J16.17, U36.4; no longer J11.17, U31.4
- net COPI6: now also J19.17, U43.4; no longer J13.17, U37.4
- net COPI7: now also J22.17, U50.4; no longer J15.17, U43.4
- net CS1: now also U6.2; no longer U7.2
- net CS2: now also J7.19, U15.2; no longer J5.19, U13.2
- net CS3: now also J10.19, U22.2; no longer J7.19, U19.2
- net CS4: now also J13.19, U29.2; no longer J9.19, U25.2
- net CS5: now also J16.19, U36.2; no longer J11.19, U31.2
- net CS6: now also J19.19, U43.2; no longer J13.19, U37.2
- net CS7: now also J22.19, U50.2; no longer J15.19, U43.2
- net FLSH_CEN: now also J5.5
- net FLSH_CEN1: now also J6.5, U12.1, U6.15; no longer U11.1, U7.15
- net FLSH_CEN2: now also J9.5, U15.15, U19.1; no longer U13.15, U17.1
- net FLSH_CEN3: now also J12.5, U22.15, U26.1; no longer U19.15, U23.1
- net FLSH_CEN4: now also J15.5, U29.15, U33.1; no longer U25.15, U29.1
- net FLSH_CEN5: now also J18.5, U36.15, U40.1; no longer U31.15, U35.1
- net FLSH_CEN6: now also J21.5, U43.15, U47.1; no longer U37.15, U41.1
- net FLSH_CEN7: now also J24.5, U50.15, U54.1; no longer U43.15, U47.1
- net FLSH_SCLK: now also J5.3
- net FLSH_SCLK1: now also J6.3, U12.6, U6.12; no longer U11.6, U7.12
- net FLSH_SCLK2: now also J9.3, U15.12, U19.6; no longer U13.12, U17.6
- net FLSH_SCLK3: now also J12.3, U22.12, U26.6; no longer U19.12, U23.6
- net FLSH_SCLK4: now also J15.3, U29.12, U33.6; no longer U25.12, U29.6
- net FLSH_SCLK5: now also J18.3, U36.12, U40.6; no longer U31.12, U35.6
- net FLSH_SCLK6: now also J21.3, U43.12, U47.6; no longer U37.12, U41.6
- net FLSH_SCLK7: now also J24.3, U50.12, U54.6; no longer U43.12, U47.6
- net FLSH_SI: now also J5.4
- net FLSH_SI1: now also J6.4, U12.5, U6.13; no longer U11.5, U7.13
- net FLSH_SI2: now also J9.4, U15.13, U19.5; no longer U13.13, U17.5
- net FLSH_SI3: now also J12.4, U22.13, U26.5; no longer U19.13, U23.5
- net FLSH_SI4: now also J15.4, U29.13, U33.5; no longer U25.13, U29.5
- net FLSH_SI5: now also J18.4, U36.13, U40.5; no longer U31.13, U35.5
- net FLSH_SI6: now also J21.4, U43.13, U47.5; no longer U37.13, U41.5
- net FLSH_SI7: now also J24.4, U50.13, U54.5; no longer U43.13, U47.5
- net FLSH_SO: now also J5.1
- net FLSH_SO1: now also J6.1, U12.2, U6.14; no longer U11.2, U7.14
- net FLSH_SO2: now also J9.1, U15.14, U19.2; no longer U13.14, U17.2
- net FLSH_SO3: now also J12.1, U22.14, U26.2; no longer U19.14, U23.2
- net FLSH_SO4: now also J15.1, U29.14, U33.2; no longer U25.14, U29.2
- net FLSH_SO5: now also J18.1, U36.14, U40.2; no longer U31.14, U35.2
- net FLSH_SO6: now also J21.1, U43.14, U47.2; no longer U37.14, U41.2
- net FLSH_SO7: now also J24.1, U50.14, U54.2; no longer U43.14, U47.2
- net G1: now also J3.3, JP9.1, K2.1; no longer J3.4, R29.2
- net G2: now also J7.3, JP14.1, K3.1; no longer J3.3, R28.1
- net G3: now also J10.3, JP19.1, K4.1; no longer J5.4, R44.2
- net G4: now also J13.3, JP24.1, K5.1; no longer J5.3, R43.1
- net G5: now also J16.3, JP29.1, K6.1; no longer J7.4, R59.2
- net G6: now also J19.3, JP34.1, K7.1; no longer J7.3, R58.1
- net G7: now also J22.3, JP39.1, K8.1; no longer J9.4, R74.2
- net G8: now also JP7.1, K1.1; no longer R10.1
- net GND: now also C46.2, C47.2, C48.2, J5.6, JP6.1, K1.2, K1.3, R1.1, R10.1, R16.1, U7.2, U8.2; no longer U6.2, U6.4, U6.5, U6.7
- net GND1: now also C70.2, C74.2, C75.2, C76.2, C80.1, C81.1, C82.1, C83.2, C86.1, C87.2, C90.1, C91.2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; no longer C49.2, C50.2, C51.2, C73.2, C76.1, C77.1, C78.1, C80.2, C81.2, C83.1, C85.2, C86.2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
- net GND2: now also C115.2, C119.2, C120.2, C122.2, C123.2, C124.2, C127.1, C129.1, C130.1, C132.2, C134.1, C136.2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; no longer C121.1, C122.1, C123.1, C124.1, C125.2, C126.2, C129.2, C130.2, C132.1, C133.2, C134.2, C94.2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
- net GND3: now also C160.2, C164.2, C165.2, C166.2, C167.2, C168.2, C172.2, C175.1, C176.1, C178.1, C182.1, C183.2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; no longer C139.2, C140.2, C141.2, C142.2, C143.2, C144.2, C145.2, C146.2, C147.2, C166.1, C167.1, C168.1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
- net GND4: now also C205.2, C209.2, C210.2, C211.2, C212.2, C213.2, C214.2, C218.2, C223.1, C224.1, C225.1, C226.1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; no longer C184.2, C185.2, C186.2, C187.2, C188.2, C189.2, C190.2, C191.2, C192.2, C193.2, C194.2, C195.2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
- net GND5: now also C250.2, C254.2, C255.2, C256.2, C257.2, C258.2, C259.2, C262.2, C263.2, C267.2, C271.1, C272.1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; no longer C229.2, C230.2, C231.2, C232.2, C233.2, C234.2, C235.2, C236.2, C237.2, C238.2, C239.2, C240.2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
- net GND6: now also C295.2, C299.2, C300.2, C301.2, C302.2, C303.2, C304.2, C307.2, C308.2, C312.2, C316.2, C319.1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; no longer C274.2, C275.2, C276.2, C277.2, C278.2, C279.2, C280.2, C281.2, C282.2, C283.2, C284.2, C285.2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
- net GND7: now also C340.2, C344.2, C345.2, C346.2, C347.2, C348.2, C349.2, C352.2, C353.2, C357.2, C362.2, C363.2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; no longer C319.2, C320.2, C321.2, C322.2, C323.2, C324.2, C325.2, C326.2, C327.2, C328.2, C329.2, C330.2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
- net INT1: now also J2.5; no longer J2.6
- net INT10: now also J13.5, U29.47; no longer J9.6, U25.47
- net INT11: now also J16.6, U36.48; no longer J11.7, U31.48
- net INT12: now also J16.5, U36.47; no longer J11.6, U31.47
- net INT13: now also J19.6, U43.48; no longer J13.7, U37.48
- net INT14: now also J19.5, U43.47; no longer J13.6, U37.47
- net INT15: now also J22.6, U50.48; no longer J15.7, U43.48
- net INT16: now also J22.5, U50.47; no longer J15.6, U43.47
- net INT2: now also J2.6; no longer J2.7
- net INT3: now also J3.6, U6.48; no longer J3.7, U7.48
- net INT4: now also J3.5, U6.47; no longer J3.6, U7.47
- net INT5: now also J7.6, U15.48; no longer J5.7, U13.48
- net INT6: now also J7.5, U15.47; no longer J5.6, U13.47
- net INT7: now also J10.6, U22.48; no longer J7.7, U19.48
- net INT8: now also J10.5, U22.47; no longer J7.6, U19.47
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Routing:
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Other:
- board size 113 x 122.2 mm -> 113 x 116.3 mm
- board text added: "X02"
- board text removed: "X01"
